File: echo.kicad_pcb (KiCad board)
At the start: 4 copper layers, 99.5 x 65 mm, 209 parts, among them J1 USB4215-03-A, J2 USB4215-03-A, J3 MDC-036, J4 DC3RX19JA2, J5 0475710001, J6 PJ-320D, J7 MDC-036, J8 SS-52100-004, Q1 BSS138, Q2 BSS138, Q3 AO3400A, Q4 AO3400A, Q5 BC850, Q6 BC850, Q7 AO3400A, Q8 AO3400A, U1 SN74CBT3257CDR, U10 AMS1117-3.3, U11 AMS1117-1.8, U12 RP2040, U13 W25Q128JVSIQ, U14 MW7211A, U15 TS3USB221RSER, U2 CH340C, U3 USBLC6-2SC6, U4 USBLC6-2SC6, U5 NCP1117 3.3, U6 W25Q32JVSIQ, U7 ESP32-D0WD, U8 ESP-PSRAM32, U9 MS9288A, X1 24.576 MHz, Y1 40 MHz, Y2 12 MHz

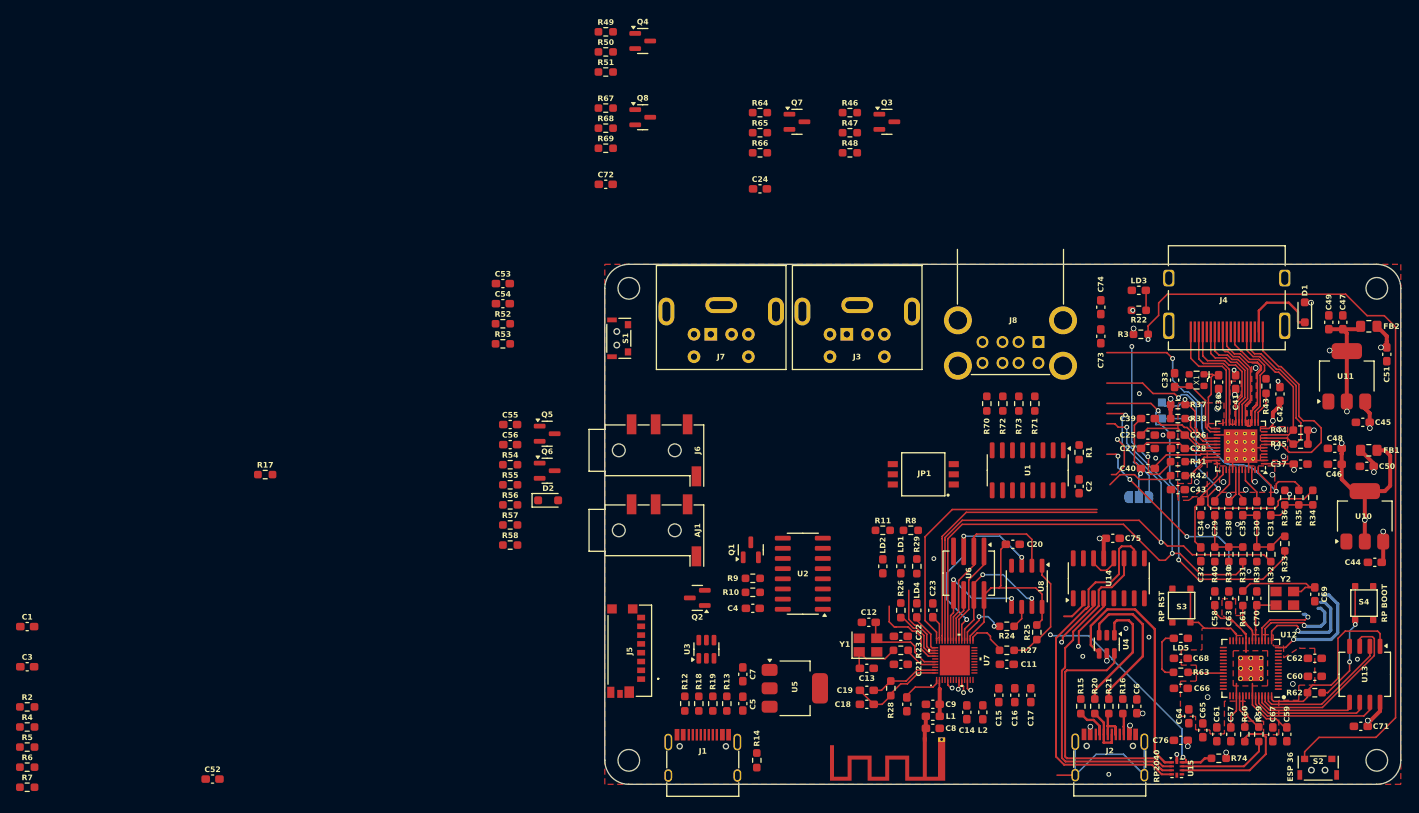
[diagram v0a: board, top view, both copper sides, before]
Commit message: Update echo.kicad_pcb
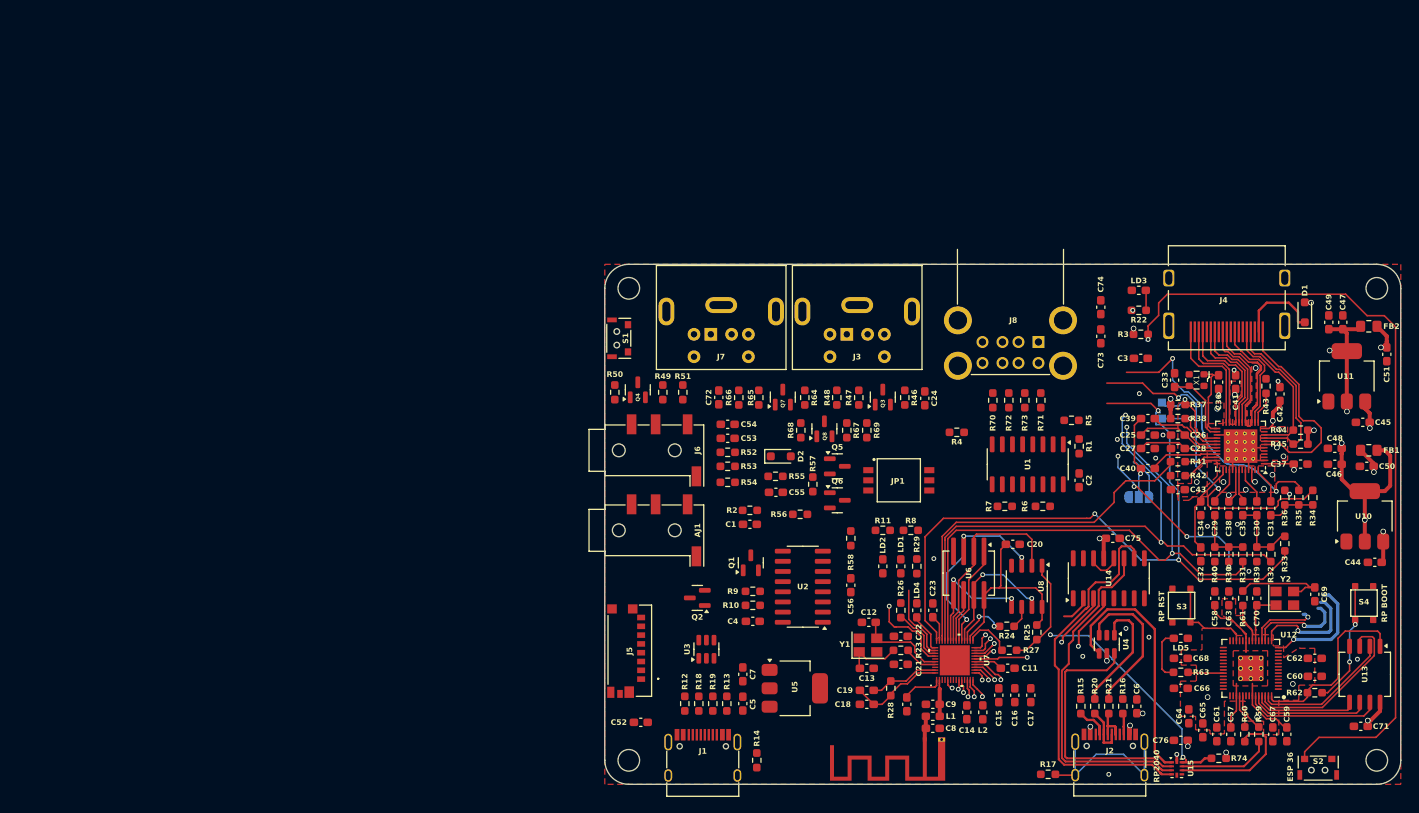
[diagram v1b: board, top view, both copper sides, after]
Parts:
- moved C3 144.4 mm to (210.2, 57.2), turned to 180 degrees
- moved R5 136.8 mm to (201.6, 65.0)
- moved R6 131.1 mm to (198.0, 75.8), turned to 180 degrees
- moved R7 127.1 mm to (193.2, 75.8), turned to 180 degrees
- moved R4 121.9 mm to (187.2, 66.5), turned to 180 degrees
- moved R17 104.8 mm to (198.7, 109.2), turned to 180 degrees
- moved R2 93.6 mm to (161.4, 76.2), turned to 180 degrees
- moved C1 91.2 mm to (161.4, 78.0)
- moved C52 54.0 mm to (147.8, 102.8)
- moved R67 50.3 mm to (173.5, 66.2), turned to -90 degrees
- moved R69 48.0 mm to (176.0, 66.2), turned to 90 degrees
- moved C56 46.1 mm to (174.0, 85.6), turned to -90 degrees
- moved R49 45.6 mm to (150.5, 61.5), turned to -90 degrees
- moved Q8 45.1 mm to (170.7, 66.1), turned to 90 degrees
- moved R68 45.0 mm to (167.8, 66.2), turned to -90 degrees
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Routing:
- net /ESP_IO19: track 80.4 -> 92.7 mm, vias 2 -> 3
- net /ESP_IO23: track 53.9 -> 46.4 mm, vias 2 -> 0
- net /ESP_IO13: track 0.00 -> 6.68 mm, vias 0 -> 1
- net /ESP_IO15: track 8.20 -> 2.66 mm, vias 0 -> 1
- net /ESP_IO12: track 0.00 -> 4.28 mm, vias 0 -> 1
- net Net-(U7-VDD3P3_RTC): track 0.00 -> 3.63 mm
- net /ESP_IO5: track 75.6 -> 72.3 mm
- net /ESP_IO14: track 0.00 -> 3.22 mm, vias 0 -> 1
- net /ESP_IO18: track 77.2 -> 74.1 mm
- net /ESP_IO0: track 0.00 -> 2.96 mm, vias 0 -> 1
- net /ESP_IO2: track 5.76 -> 3.00 mm, vias 1 -> 2
- net /ESP_IO25: track 0.00 -> 2.61 mm, vias 0 -> 1
- net /ESP_IO27: track 0.00 -> 2.41 mm, vias 0 -> 1
- net /ESP_IO33: track 0.00 -> 2.32 mm, vias 0 -> 1
- net /ESP_IO22: track 41.4 -> 39.4 mm
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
